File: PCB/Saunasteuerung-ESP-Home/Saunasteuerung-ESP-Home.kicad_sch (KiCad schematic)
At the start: 17 parts, among them J5 I2C, J7 WS2812, Q10 2N7002, U5 DS18B20, X1 Sensors

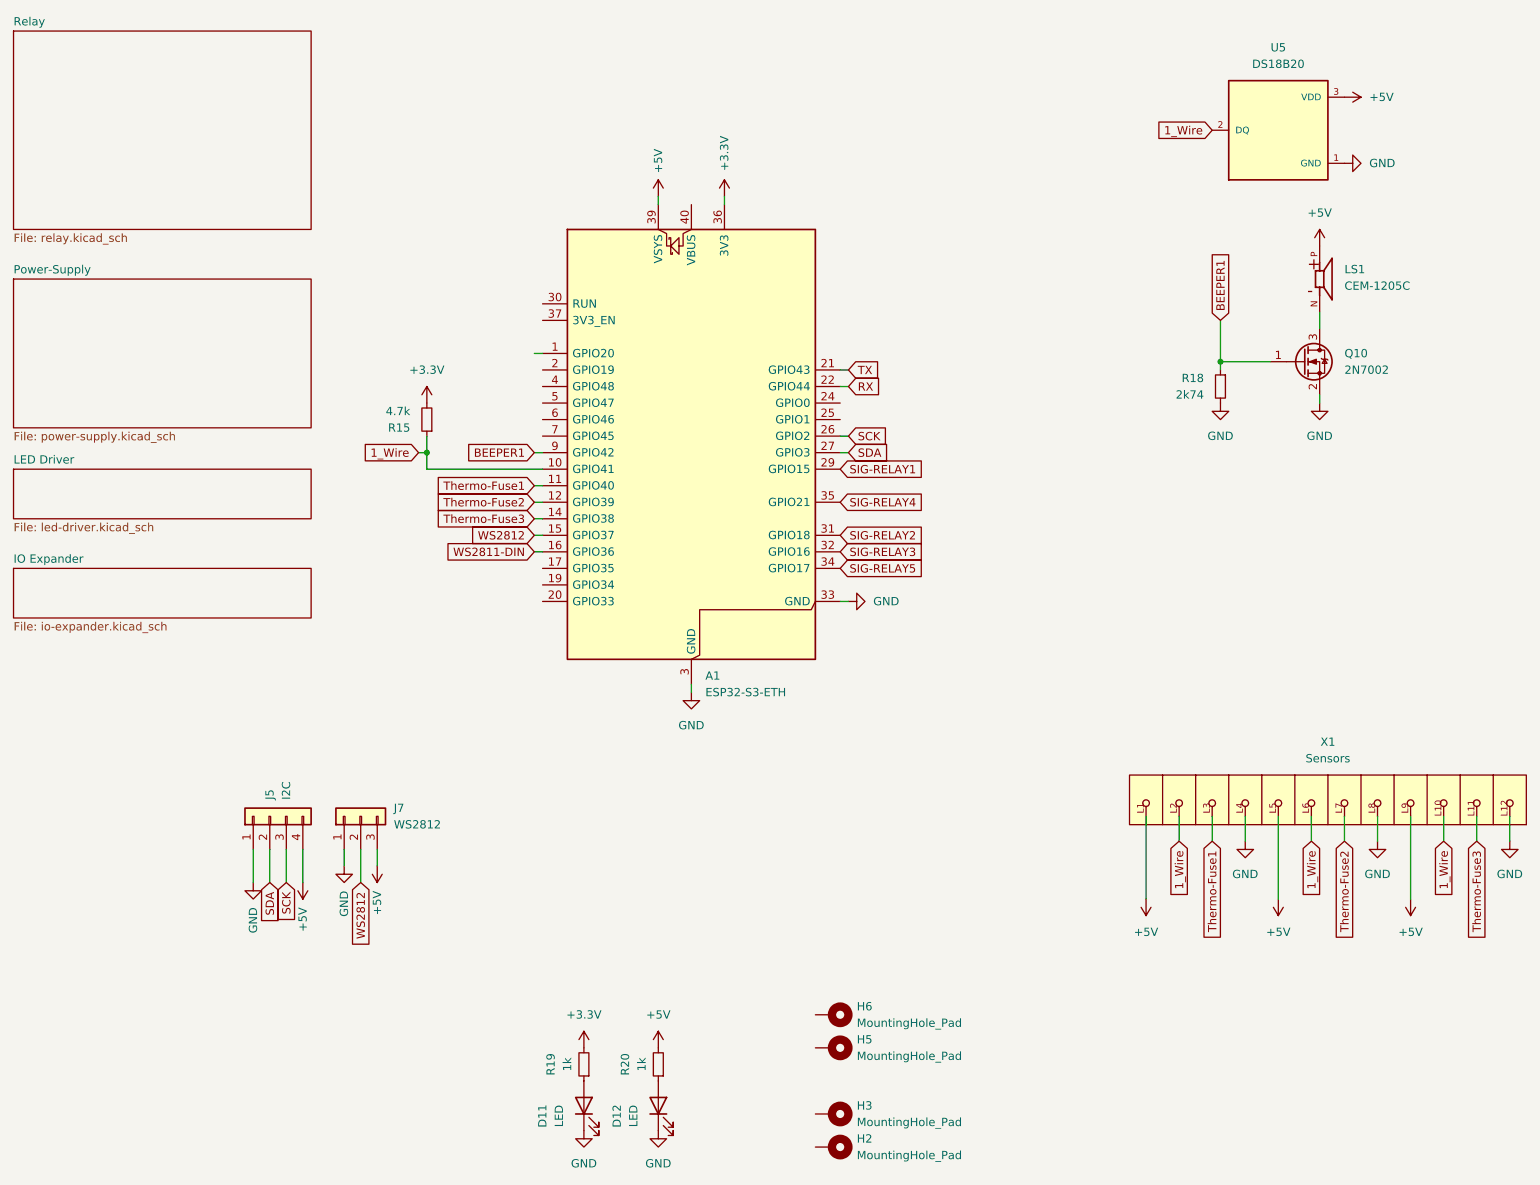
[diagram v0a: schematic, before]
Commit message: update
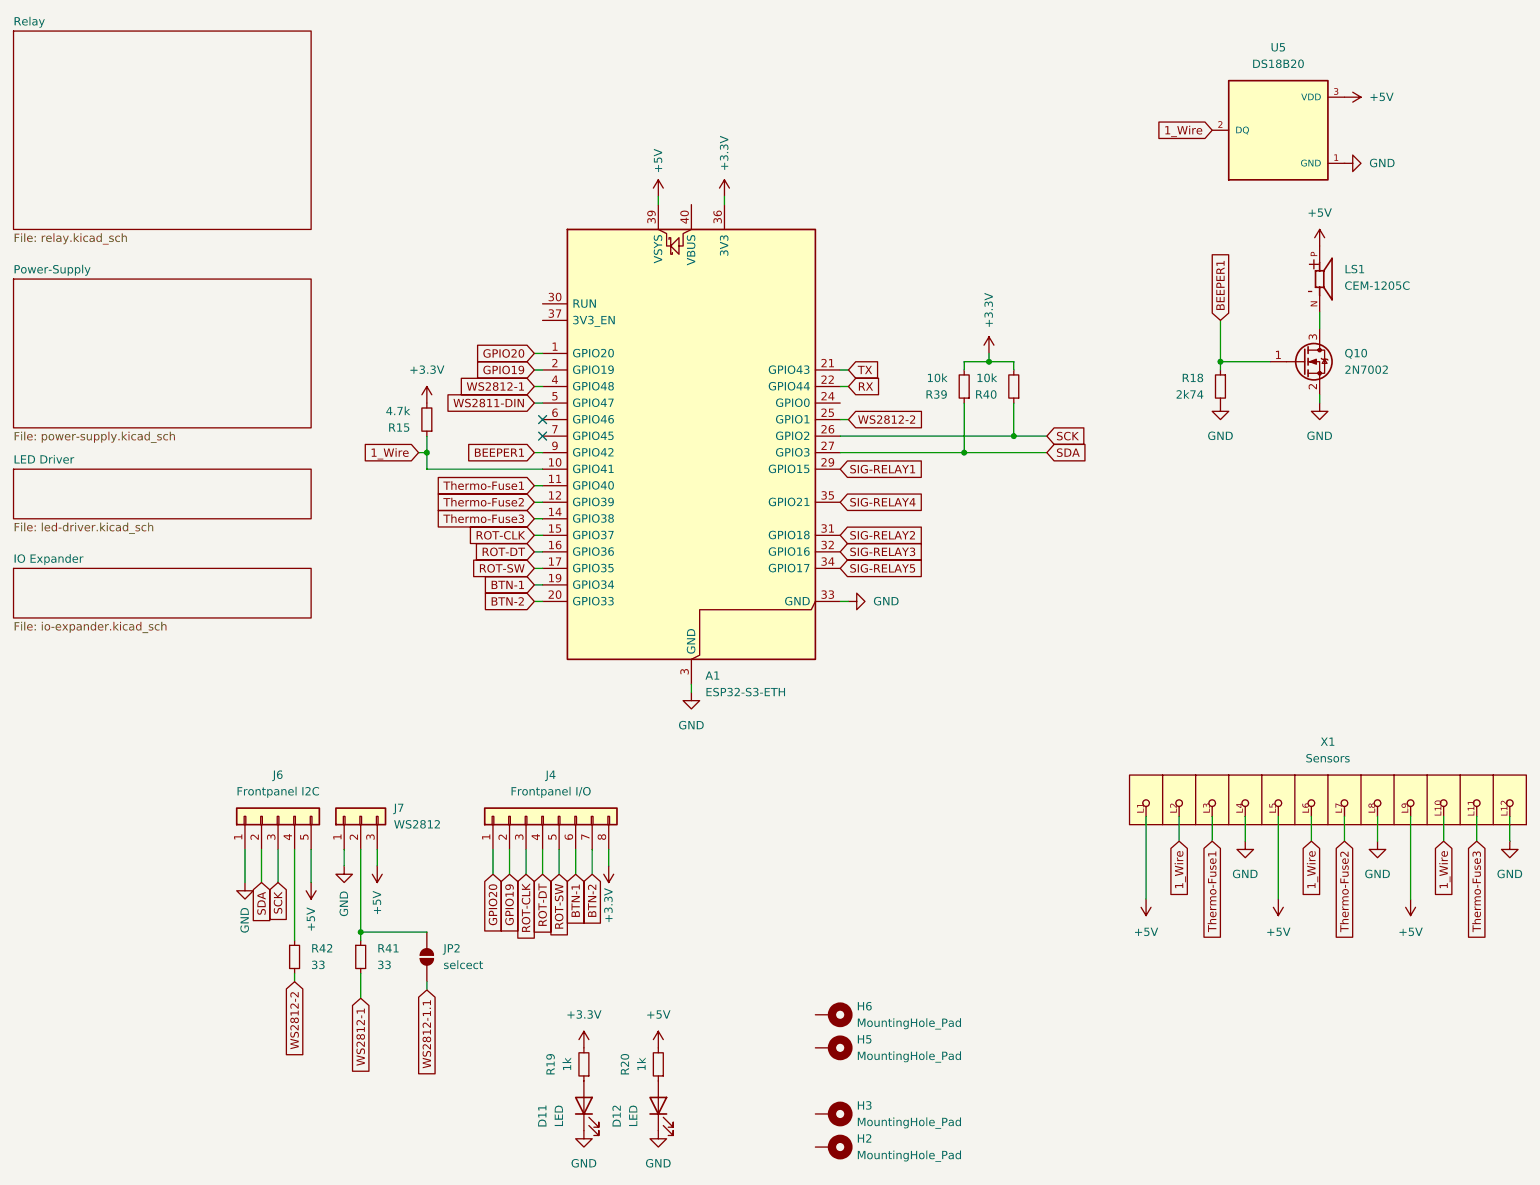
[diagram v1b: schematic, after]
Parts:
- removed J5: I2C, Connector_JST:JST_XH_B4B-XH-A_1x04_P2.50mm_Vertical, symbol Connector_Generic:Conn_01x04
- added J4: Frontpanel I/O, Connector_JST:JST_XH_B8B-XH-A_1x08_P2.50mm_Vertical, symbol Connector_Generic:Conn_01x08
- added J6: Frontpanel I2C, Connector_JST:JST_XH_B5B-XH-A_1x05_P2.50mm_Vertical, symbol Connector_Generic:Conn_01x05
- added JP2: selcect, Jumper:SolderJumper-2_P1.3mm_Open_TrianglePad1.0x1.5mm, symbol Jumper:SolderJumper_2_Open
- added R39, R40: 10k, Resistor_SMD:R_0603_1608Metric, symbol Device:R_Small
- added R41, R42: 33, Resistor_SMD:R_0603_1608Metric, symbol Device:R_Small
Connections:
- net +3.3V: now also J4.8 (Pin_8), R39.2, R40.2
- net +5V: now also J6.5 (Pin_5)
- net GND: now also J6.1 (Pin_1)
- net SCK: now also J6.3 (Pin_3), R40.1
- net SDA: now also J6.2 (Pin_2), R39.1
- net WS2811-DIN: now also A1.5 (GPIO47); no longer A1.16 (GPIO36)
- net GPIO20: now reaches A1.1 (GPIO20)
- net GPIO20: now also J4.1 (Pin_1)
- net ROT-SW: now reaches A1.17 (GPIO35)
- net ROT-SW: now also J4.5 (Pin_5)
- net BTN-1: now reaches A1.19 (GPIO34)
- net BTN-1: now also J4.6 (Pin_6)
- net GPIO19: now reaches A1.2 (GPIO19)
- net GPIO19: now also J4.2 (Pin_2)
- net BTN-2: now reaches A1.20 (GPIO33)
- net BTN-2: now also J4.7 (Pin_7)
- net WS2812-2: now reaches A1.25 (GPIO1)
- net WS2812-2: now also R42.2
- net WS2812-1: now reaches A1.4 (GPIO48)
- net WS2812-1: now also R41.2
- net WS2812: no longer names the net of J7.2 (Pin_2)
- net WS2812: now also JP2.2 (B), R41.1; no longer A1.15 (GPIO37)
- new net: J6.4 (Pin_4), R42.1
- new net ROT-CLK: A1.15 (GPIO37), J4.3 (Pin_3)
- new net ROT-DT: A1.16 (GPIO36), J4.4 (Pin_4)
- new net WS2812-1.1: JP2.1 (A)
- no-connect marks 0 -> 2
